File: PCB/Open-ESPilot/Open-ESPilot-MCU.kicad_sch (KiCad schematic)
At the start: 15 parts, among them J1 USB_C_Receptacle_USB2.0_16P, SW1 SW_Push, SW2 SW_Push, U1 ESP32-S3-WROOM-1-N8

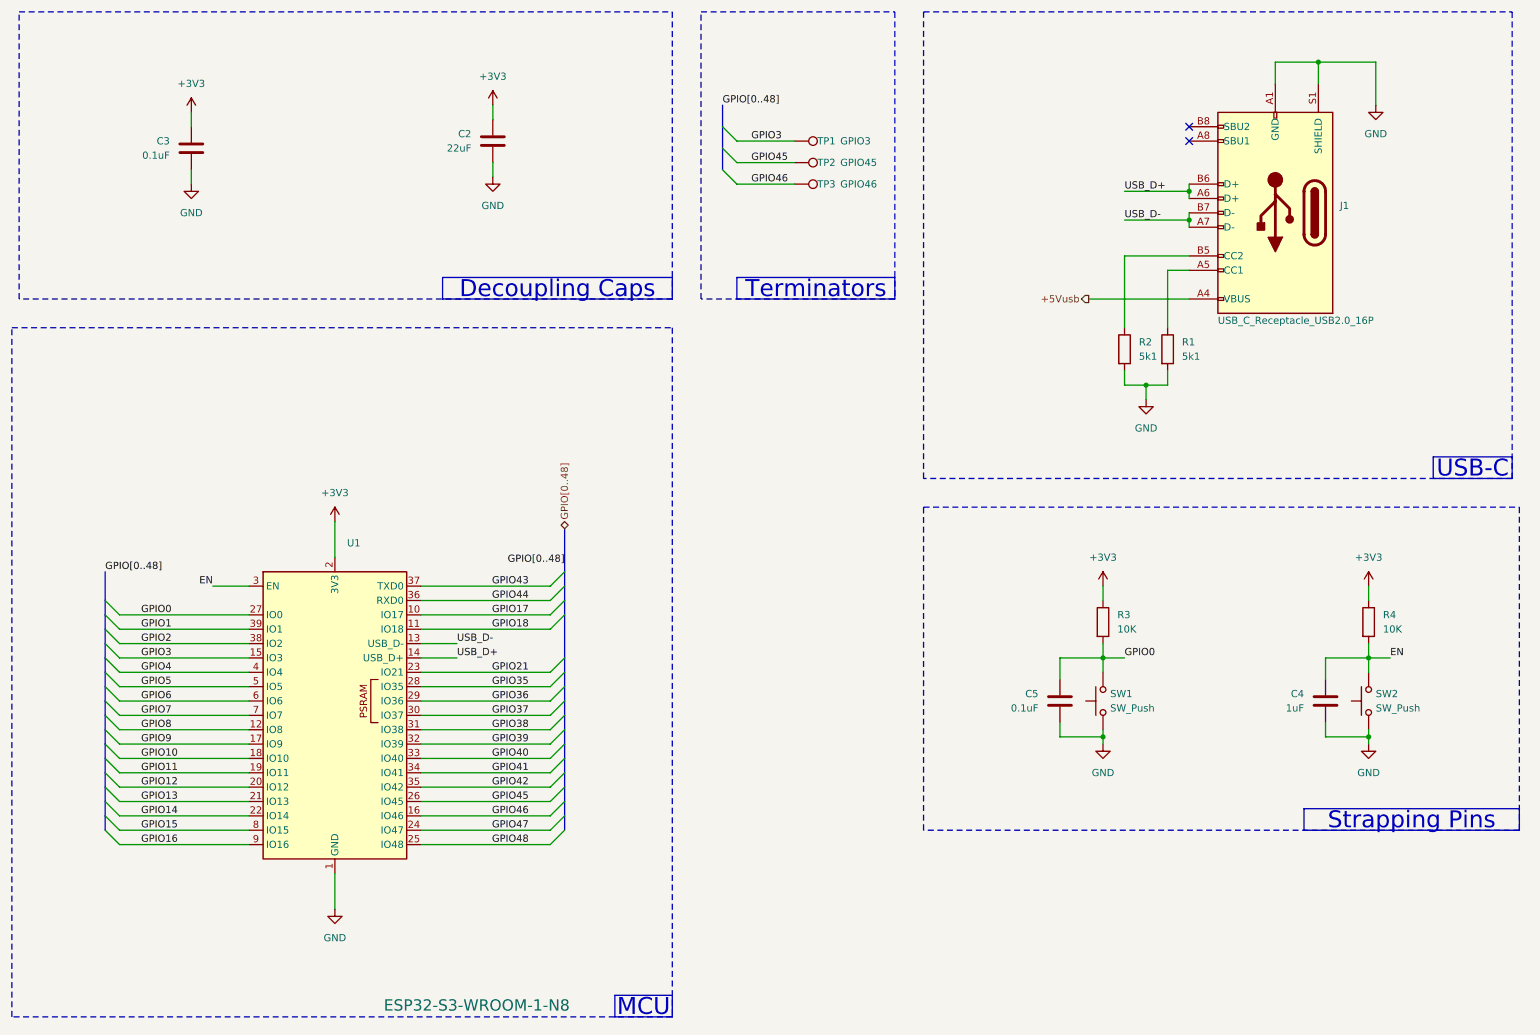
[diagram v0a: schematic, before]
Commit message: more Schematic fixes yay
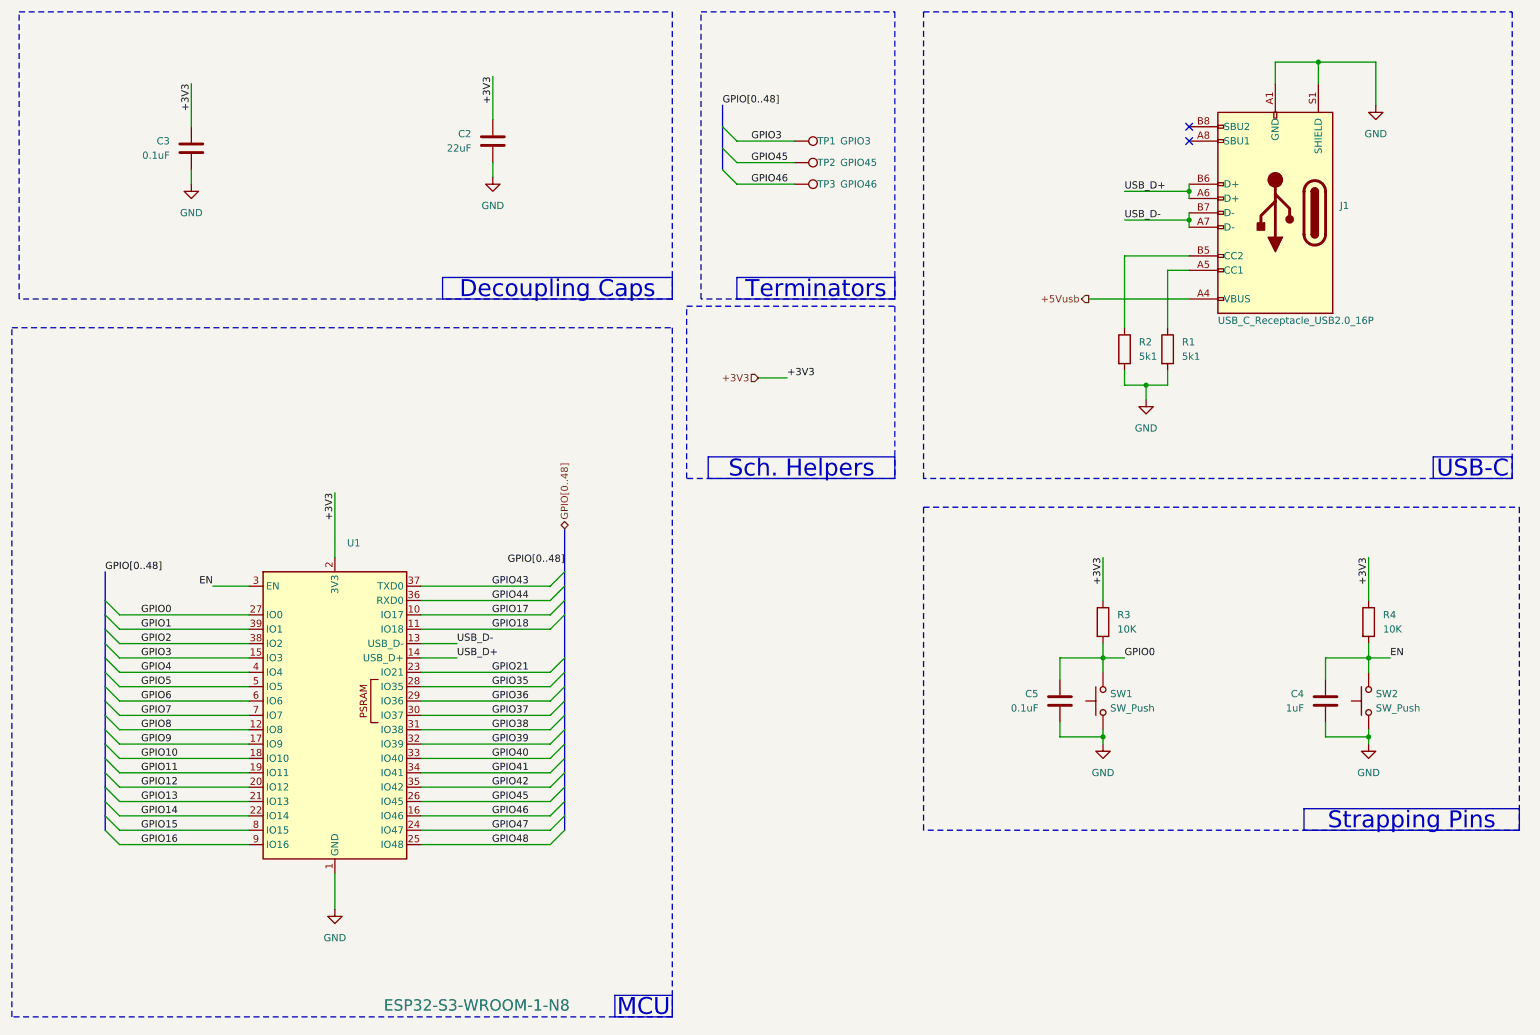
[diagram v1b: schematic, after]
